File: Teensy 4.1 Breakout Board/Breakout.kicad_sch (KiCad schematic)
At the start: 16 parts, among them J1 CAN1, J2 CAN2, J3 12V_IN, J4 APPS, J5 BRAKE_PRESSURE_IN, J6 BRAKE_LIGHT_OUT, J7 3.3V_OUT, J8 GND_COMMON, Q1 IRLZ44N, U1 Teensy4.1, U2 MCP2562-E-P, U3 LM2596S-5, U4 MCP2562-E-P

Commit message: breakout board v1 sizing
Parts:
- removed J1: CAN1, TerminalBlock_Phoenix:TerminalBlock_Phoenix_MKDS-1,5-2-5.08_1x02_P5.08mm_Horizontal, symbol Connector:Screw_Terminal_01x02
- removed J2: CAN2, TerminalBlock_Phoenix:TerminalBlock_Phoenix_MKDS-1,5-2-5.08_1x02_P5.08mm_Horizontal, symbol Connector:Screw_Terminal_01x02
- removed J3: 12V_IN, TerminalBlock_Phoenix:TerminalBlock_Phoenix_MKDS-1,5-2-5.08_1x02_P5.08mm_Horizontal, symbol Connector:Screw_Terminal_01x02
- removed J4: APPS, TerminalBlock_Phoenix:TerminalBlock_Phoenix_MKDS-1,5-2-5.08_1x02_P5.08mm_Horizontal, symbol Connector:Screw_Terminal_01x02
- removed J5: BRAKE_PRESSURE_IN, TerminalBlock_Phoenix:TerminalBlock_Phoenix_MKDS-1,5-2-5.08_1x02_P5.08mm_Horizontal, symbol Connector:Screw_Terminal_01x02
- removed J6: BRAKE_LIGHT_OUT, TerminalBlock_Phoenix:TerminalBlock_Phoenix_MKDS-1,5-2-5.08_1x02_P5.08mm_Horizontal, symbol Connector:Screw_Terminal_01x02
- removed J7: 3.3V_OUT, TerminalBlock_Phoenix:TerminalBlock_Phoenix_MKDS-1,5-4-5.08_1x04_P5.08mm_Horizontal, symbol Connector:Screw_Terminal_01x04
- removed J8: GND_COMMON, TerminalBlock_Phoenix:TerminalBlock_Phoenix_MKDS-1,5-4-5.08_1x04_P5.08mm_Horizontal, symbol Connector:Screw_Terminal_01x04
- removed Q1: IRLZ44N, Package_TO_SOT_THT:TO-220-3_Vertical, symbol Transistor_FET:IRLZ44N
- removed U1: Teensy4.1, teensy:Teensy41, symbol teensy:Teensy4.1
- removed U2, U4: MCP2562-E-P, Package_DIP:DIP-8_W7.62mm, symbol Interface_CAN_LIN:MCP2562-E-P
- removed U3: LM2596S-5, Package_TO_SOT_SMD:TO-263-5_TabPin3, symbol Regulator_Switching:LM2596S-5
- added C1, C2, C3, C5, C6, C7, C8: 0.1uF, FA14_Capacitor:FA18X7R1H104KNU00, symbol Device:C
- added C15: 220uF, Capacitor_THT:CP_Radial_D6.3mm_P2.50mm, symbol Device:C_Polarized
- added C18: 680uF, footprints:CAPPRD500W60D1275H2700, symbol 50ZLJ680M12_5X25:50ZLJ680M12.5X25
- added C9: 10uF, Capacitor_THT:CP_Radial_D5.0mm_P2.50mm, symbol Device:C_Polarized
- added D1: NUP3105L, Package_TO_SOT_SMD:SOT-23, symbol Power_Protection:NUP2105L
- added D3: 1N5821, Diode_THT:D_DO-201AD_P15.24mm_Horizontal, symbol Diode:1N5821
- added J1: CAN, Connector_JST:JST_XH_B3B-XH-A_1x03_P2.50mm_Vertical, symbol Connector_Generic:Conn_01x03
- added J10: RTD_Speaker, Connector_JST:JST_XH_B2B-XH-A_1x02_P2.50mm_Vertical, symbol Connector_Generic:Conn_01x02
- added J2: 12V Power, Connector_JST:JST_XH_B2B-XH-A_1x02_P2.50mm_Vertical, symbol Connector_Generic:Conn_01x02
- added J3: APPS1, Connector_JST:JST_XH_B3B-XH-A_1x03_P2.50mm_Vertical, symbol Connector_Generic:Conn_01x03
- added J4: APPS2, Connector_JST:JST_XH_B3B-XH-A_1x03_P2.50mm_Vertical, symbol Connector_Generic:Conn_01x03
- added J5: Brake_Pressure_Front, Connector_JST:JST_XH_B3B-XH-A_1x03_P2.50mm_Vertical, symbol Connector_Generic:Conn_01x03
- added J6: Brake_Pressure_Rear, Connector_JST:JST_XH_B3B-XH-A_1x03_P2.50mm_Vertical, symbol Connector_Generic:Conn_01x03
- added J7: Nextion, Connector_JST:JST_XH_B4B-XH-A_1x04_P2.50mm_Vertical, symbol Connector_Generic:Conn_01x04
- added J8: ESP32, Connector_JST:JST_XH_B4B-XH-A_1x04_P2.50mm_Vertical, symbol Connector_Generic:Conn_01x04
- added J9: Brake_Light, Connector_JST:JST_XH_B2B-XH-A_1x02_P2.50mm_Vertical, symbol Connector_Generic:Conn_01x02
- added JP1: SolderJumper_2_Open, Jumper:SolderJumper-2_P1.3mm_Open_Pad1.0x1.5mm, symbol Jumper:SolderJumper_2_Open
- added L1: 33uH, Inductor_SMD:L_10.4x10.4_H4.8, symbol Device:L
- added Q1, Q2: 2N7000, Package_TO_SOT_THT:TO-92_Inline, symbol Transistor_FET:2N7000
- added R10, R12, R4: 20k, Resistor_THT:R_Axial_DIN0207_L6.3mm_D2.5mm_P10.16mm_Horizontal, symbol Device:R
- added R11, R9: 10k, Resistor_THT:R_Axial_DIN0207_L6.3mm_D2.5mm_P10.16mm_Horizontal, symbol Device:R
- added R13, R14, R15, R16: 1k, Resistor_THT:R_Axial_DIN0207_L6.3mm_D2.5mm_P10.16mm_Horizontal, symbol Device:R
- added R5, R7: 100, Resistor_THT:R_Axial_DIN0207_L6.3mm_D2.5mm_P10.16mm_Horizontal, symbol Device:R
- added R6, R8: 100k, Resistor_THT:R_Axial_DIN0207_L6.3mm_D2.5mm_P10.16mm_Horizontal, symbol Device:R
- added R_CAN_TERM1: 120, Resistor_THT:R_Axial_DIN0207_L6.3mm_D2.5mm_P10.16mm_Horizontal, symbol Device:R
- added U1: SN65HVD230, Package_SO:SOIC-8_3.9x4.9mm_P1.27mm, symbol Interface_CAN_LIN:SN65HVD230
- added U2: module_mpu6050, usini_sensors:module_mpu6050, symbol usini_sensors:module_mpu6050
- added U26: LM2596SX-5.0/NOPB, Package_TO_SOT_SMD:TO-263-5_TabPin3, symbol Regulator_Switching:LM2596S-5
- added U3: Teensy4.1, teensy.pretty-master:Teensy41, symbol teensy:Teensy4.1
- R1: value 120 -> 10k; footprint Resistor_SMD:R_0603_1608Metric -> Resistor_THT:R_Axial_DIN0207_L6.3mm_D2.5mm_P10.16mm_Horizontal; Part Number (none) -> MCF 0.25W 10K
- R2: value 120 -> 20k; footprint Resistor_SMD:R_0603_1608Metric -> Resistor_THT:R_Axial_DIN0207_L6.3mm_D2.5mm_P10.16mm_Horizontal; Part Number (none) -> CFR25SJT-52A20K
- R3: value 10K -> 10k; footprint Resistor_SMD:R_0603_1608Metric -> Resistor_THT:R_Axial_DIN0207_L6.3mm_D2.5mm_P10.16mm_Horizontal; Part Number (none) -> MCF 0.25W 10K
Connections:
- net 3.3V: now also C1.2, C2.2, U1.3 (VCC), U2.1 (VCC), U3.46 (3V3)
- net 5V: now also C15.1, C3.2, C9.1, J3.1 (Pin_1), J4.1 (Pin_1), J5.1 (Pin_1), J6.1 (Pin_1), J7.1 (Pin_1), J8.1 (Pin_1), L1.2, U26.4 (FB), U3.48 (VIN)
- net APPS1: now also R1.1, J3.2 (Pin_2)
- net APPS2: now also R3.1, J4.2 (Pin_2)
- net CAN1_RX: now also U1.4 (R), U3.45 (23_A9_CRX1_MCLK1)
- net CAN1_TX: now also U1.1 (D), U3.44 (22_A8_CTX1)
- net GND: now also R2.2, C1.1, C15.2, C18.2 (-), C2.1, C3.1, C5.2, C6.2, C7.2, C8.2, C9.2, D1.3 (A), D3.2 (A), J1.1 (Pin_1), J2.2 (Pin_2), J3.3 (Pin_3), J4.3 (Pin_3), J5.3 (Pin_3), J6.3 (Pin_3), J7.4 (Pin_4), J8.4 (Pin_4), Q1.1 (S), Q2.1 (S), R10.2, R12.2, R4.2, R6.1, R8.1, U1.2 (GND), U1.8 (Rs), U2.2 (GND), U26.3 (GND), U26.5 (~{ON}/OFF), U3.47 (GND); no longer R3.1
- net at R2.1: now also R1.2, R13.2
- net BRAKE_LIGHT_CONTROL: no longer names the net of R3.2
- net BRAKE_LIGHT_CONTROL: now also R14.2, R4.1
- new net: Q1.2 (G), R5.2, R6.2
- new net: Q2.2 (G), R7.2, R8.2
- new net: JP1.2 (B), R_CAN_TERM1.2
- new net: D3.1 (K), L1.1, U26.2 (OUT)
- new net: R11.2, R12.1, R16.2
- new net: R10.1, R15.2, R9.2
- new net: J9.2 (Pin_2), Q1.3 (D)
- new net: J10.2 (Pin_2), Q2.3 (D)
- new net 12V: C18.1 (+), J10.1 (Pin_1), J2.1 (Pin_1), J9.1 (Pin_1), U26.1 (VIN)
- new net APPS1_3.3V: C5.1, R13.1, U3.36 (14_A0_TX3_SPDIF_OUT)
- new net APPS2_3.3V: C6.1, R14.1, U3.37 (15_A1_RX3_SPDIF_IN)
- new net Brake_Front: J5.2 (Pin_2), R9.1
- new net Brake_Front_3.3V: C7.1, R15.1, U3.38 (16_A2_RX4_SCL1)
- new net Brake_Light_EN: R5.1, U3.8 (6_OUT1D)
- new net Brake_Rear: J6.2 (Pin_2), R11.1
- new net Brake_Rear_3.3V: C8.1, R16.1, U3.39 (17_A3_TX4_SDA1)
- new net CANH: D1.1 (K), J1.3 (Pin_3), R_CAN_TERM1.1, U1.7 (CANH)
- new net CANL: D1.2 (K), J1.2 (Pin_2), JP1.1 (A), U1.6 (CANL)
- new net ESP32_RX: J8.3 (Pin_3), U3.10 (8_TX2_IN1)
- new net ESP32_TX: J8.2 (Pin_2), U3.9 (7_RX2_OUT1A)
- new net MPU_SCL: U2.3 (SCL), U3.41 (19_A5_SCL)
- new net MPU_SDA: U2.4 (SDA), U3.40 (18_A4_SDA)
- new net Nextion_RX: J7.3 (Pin_3), U3.3 (1_TX1_CTX2_MISO1)
- new net Nextion_TX: J7.2 (Pin_2), U3.2 (0_RX1_CRX2_CS1)
- new net RTD_Speaker_EN: R7.1, U3.11 (9_OUT1C)
- no-connect marks 1 -> 2
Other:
- note added: "120 Ω CAN termination Populate only if this PCB is end-of-bus"
- note added: "Analogue Sensors"
- note added: "Assuming M7100, and scaling down to 3.3V"
- note added: "Brake Light and Speaker"
- note added: "Buck Converter"
- note added: "CAN TVS Protection Diode"
- note added: "CAN Transceiver"
- note added: "Consider replacing for synchronous buck and different output based on current requirements"
- note added: "ESP32 TX to Teensy RX Teensy TX to ESP32 RX"
- note added: "LP Filter should be physically close to Teensy"
- note added: "MPU Sensor"
- note added: "Nextion TX to Teensy RX Teensy TX to Nextion RX"
- note added: "Pin 1: Red wire Pin 2: Black Wire"
- note added: "RS to GND for High Speed mode"
- note added: "Serial 1"
- note added: "Serial 2"
- note added: "Teensy 4.1 Microcontroller"
- note added: "UART Interface"
- note added: "VIN and VUSB link on Teensy 4.1 should be cut to avoid back-feeding"
- note added: "Will be mounted on socket 2x24 and some others"
- note added: "all ADC signals need a return ground to prevent ground offset and jitter. Ground locally at chassis is not a good idea"
- note added: "buck converter"
- note added: "check current"
- note added: "no pull up resistors necessary for adafruit mpu6050"
- note added: "probably need more input protection"
- note removed: "Keelan Test"

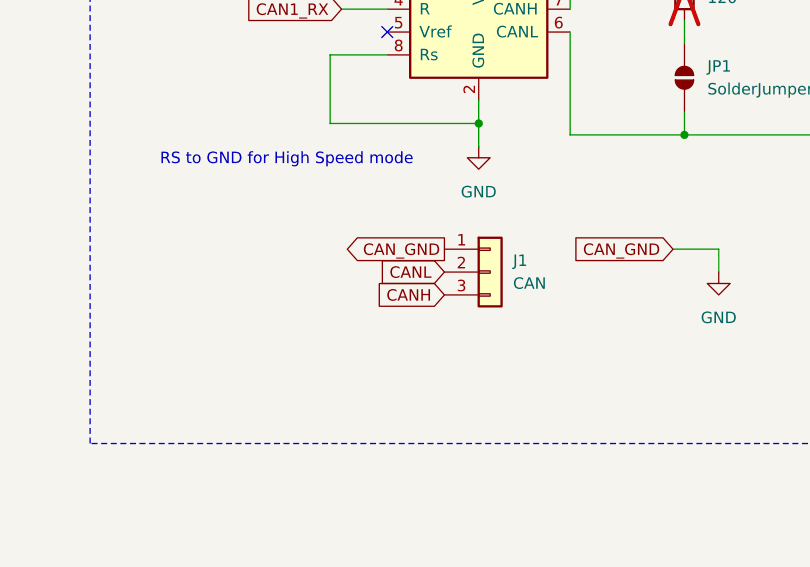
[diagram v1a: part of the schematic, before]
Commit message: breakout complete
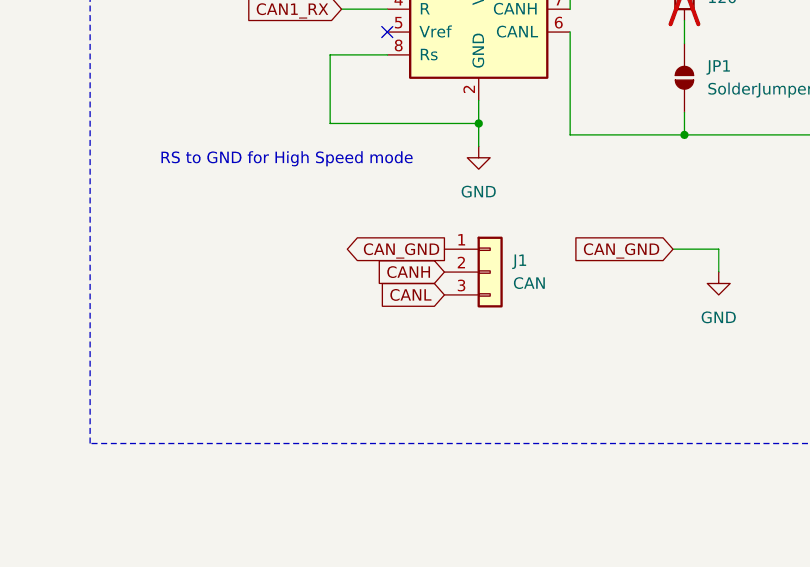
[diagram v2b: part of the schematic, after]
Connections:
- net CANH: now also J1.2 (Pin_2); no longer J1.3 (Pin_3)
- net CANL: now also J1.3 (Pin_3); no longer J1.2 (Pin_2)
